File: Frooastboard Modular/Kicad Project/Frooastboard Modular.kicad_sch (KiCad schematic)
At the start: 41 parts, among them J1 Conn_01x08, J2 Conn_01x06, J3 Conn_01x06, J4 Conn_01x10, J5 Conn_01x12, J6 SW Interface, J7 Conn_01x04, J8 Conn_01x08, U1 IS31FL3733-QF, U2 RP2040, U3 W25Q32JVZP, U4 LM317L_SOT-89, Y1 12MHz

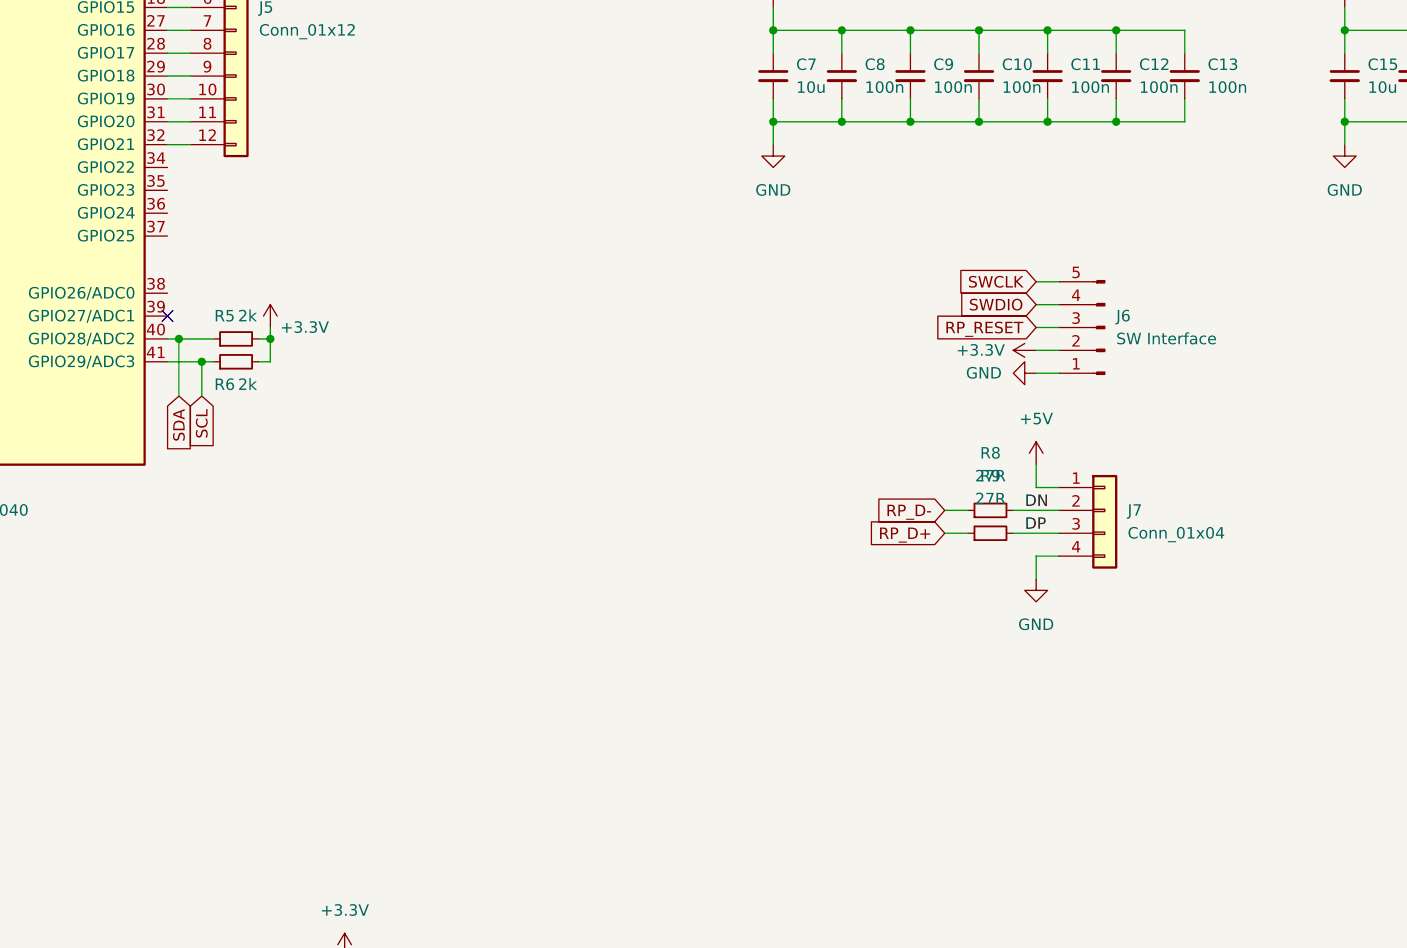
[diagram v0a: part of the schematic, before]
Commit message: before moving stuff
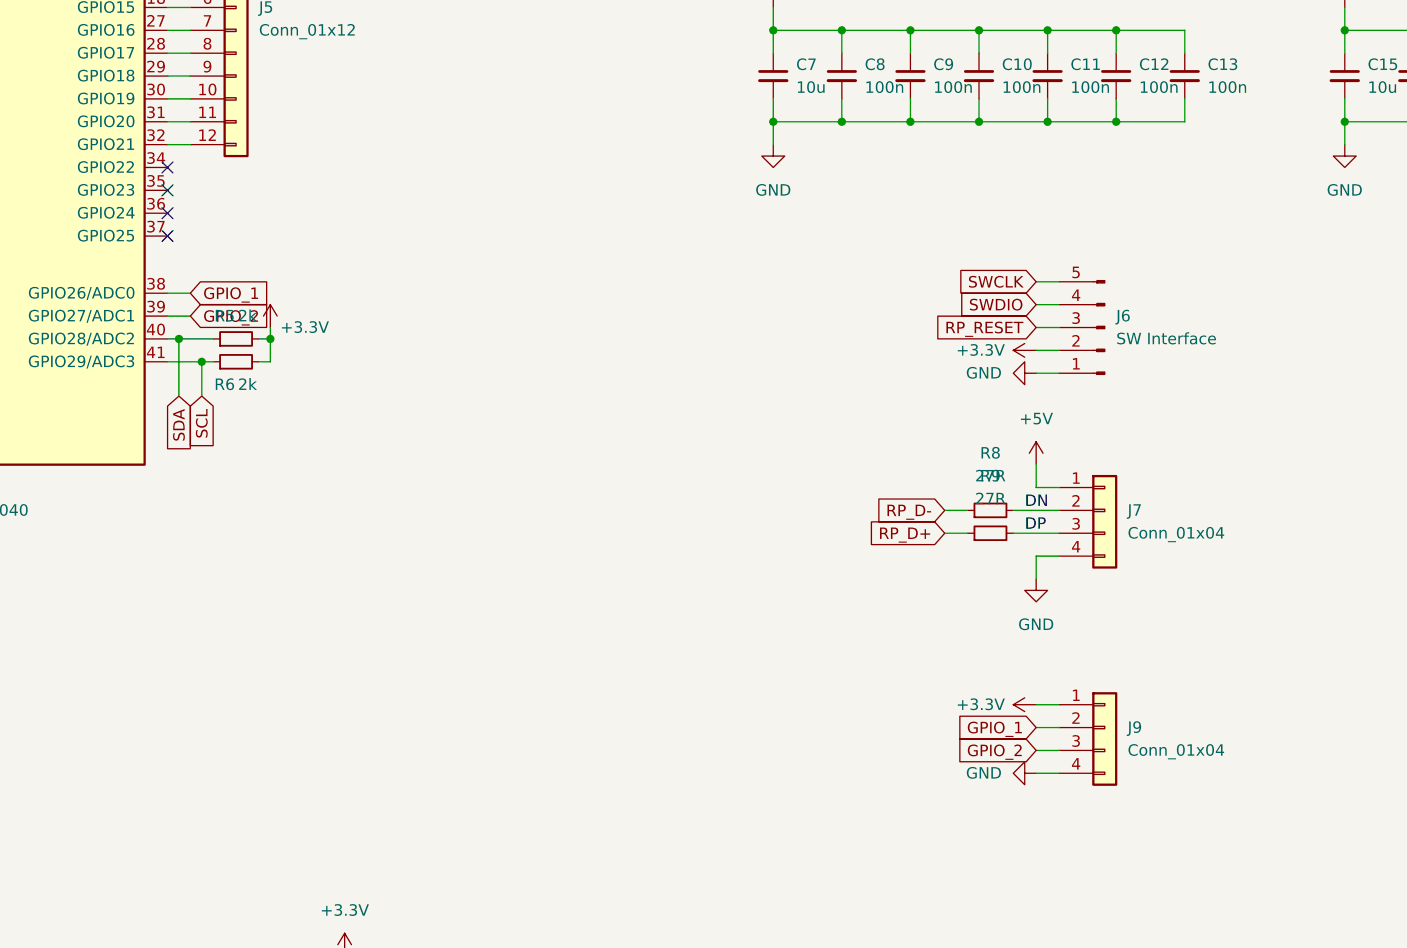
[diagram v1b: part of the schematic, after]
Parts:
- added J9: Conn_01x04, Frooastboard Footprints:PinHeader_1x04_P1.27mm_Vertical, symbol Connector_Generic:Conn_01x04
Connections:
- net +3V3: now also J9.1 (Pin_1)
- net GND: now also J9.4 (Pin_4)
- net GPIO_1: now reaches U2.38 (GPIO26/ADC0)
- net GPIO_1: now also J9.2 (Pin_2)
- net GPIO_2: now reaches U2.39 (GPIO27/ADC1)
- net GPIO_2: now also J9.3 (Pin_3)
- no-connect marks 3 -> 6
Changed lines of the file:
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@@
   (junction (at 203.2 29.21) (diameter 0) (color 0 0 0 0)
   )
+  (no_connect (at 90.17 95.25))
   (no_connect (at 48.26 199.39))
-  (no_connect (at 90.17 109.22))
+  (no_connect (at 90.17 97.79))
+  (no_connect (at 90.17 100.33))
+  (no_connect (at 90.17 92.71))
   (no_connect (at 48.26 209.55))
   (wire (pts (xy 138.43 40.64) (xy 135.89 40.64))
@@
     (stroke (width 0) (type default))
   )
+  (wire (pts (xy 90.17 106.68) (xy 92.71 106.68))
+    (stroke (width 0) (type default))
+  )
   (wire (pts (xy 66.04 128.27) (xy 66.04 130.81))
     (stroke (width 0) (type default))
@@
     (stroke (width 0) (type default))
   )
+  (wire (pts (xy 90.17 109.22) (xy 92.71 109.22))
+    (stroke (width 0) (type default))
+  )
   (wire (pts (xy 261.62 36.83) (xy 261.62 39.37))
     (stroke (width 0) (type default))
@@
     (stroke (width 0) (type default))
   )
+  (wire (pts (xy 186.69 157.48) (xy 189.23 157.48))
+    (stroke (width 0) (type default))
+  )
   (wire (pts (xy 66.04 267.97) (xy 66.04 265.43))
     (stroke (width 0) (type default))
@@
     (stroke (width 0) (type default))
   )
+  (wire (pts (xy 186.69 160.02) (xy 189.23 160.02))
+    (stroke (width 0) (type default))
+  )
   (wire (pts (xy 123.825 193.04) (xy 133.985 193.04))
     (stroke (width 0) (type default))
@@
     (stroke (width 0) (type default))
   )
+  (wire (pts (xy 186.69 154.94) (xy 189.23 154.94))
+    (stroke (width 0) (type default))
+  )
   (wire (pts (xy 135.89 40.64) (xy 135.89 43.18))
     (stroke (width 0) (type default))
@@
     (stroke (width 0) (type default))
   )
+  (wire (pts (xy 186.69 152.4) (xy 189.23 152.4))
+    (stroke (width 0) (type default))
+  )
   (wire (pts (xy 261.62 39.37) (xy 264.16 39.37))
     (stroke (width 0) (type default))
@@
     )
   )
+  (global_label "GPIO_1" (shape input) (at 186.69 154.94 180) (fields_autoplaced)
+    (effects (font (size 1.27 1.27)) (justify right))
+    (property "Intersheetrefs" "${INTERSHEET_REFS}" (at 177.1318 154.94 0)
+      (effects (font (size 1.27 1.27)) (justify right) hide)
+    )
+  )
   (global_label "QSPI_SD0" (shape input) (at 46.99 104.14 180) (fields_autoplaced)
     (effects (font (size 1.27 1.27)) (justify right))
@@
     )
   )
+  (global_label "GPIO_1" (shape input) (at 92.71 106.68 0) (fields_autoplaced)
+    (effects (font (size 1.27 1.27)) (justify left))
+    (property "Intersheetrefs" "${INTERSHEET_REFS}" (at 102.2682 106.68 0)
+      (effects (font (size 1.27 1.27)) (justify left) hide)
+    )
+  )
   (global_label "SWDIO" (shape input) (at 46.99 93.98 180) (fields_autoplaced)
     (effects (font (size 1.27 1.27)) (justify right))
@@
     )
   )
+  (global_label "GPIO_2" (shape input) (at 92.71 109.22 0) (fields_autoplaced)
+    (effects (font (size 1.27 1.27)) (justify left))
+    (property "Intersheetrefs" "${INTERSHEET_REFS}" (at 102.2682 109.22 0)
+      (effects (font (size 1.27 1.27)) (justify left) hide)
+    )
+  )
   (global_label "QSPI_SD3" (shape input) (at 46.99 111.76 180) (fields_autoplaced)
     (effects (font (size 1.27 1.27)) (justify right))
@@
     )
   )
+  (global_label "GPIO_2" (shape input) (at 186.69 157.48 180) (fields_autoplaced)
+    (effects (font (size 1.27 1.27)) (justify right))
+    (property "Intersheetrefs" "${INTERSHEET_REFS}" (at 177.1318 157.48 0)
+      (effects (font (size 1.27 1.27)) (justify right) hide)
+    )
+  )
   (global_label "SDA" (shape input) (at 45.72 194.31 180) (fields_autoplaced)
     (effects (font (size 1.27 1.27)) (justify right))
@@
     )
   )
+  (symbol (lib_id "power:GND") (at 186.69 160.02 270) (unit 1)
+    (in_bom yes) (on_board yes) (dnp no) (fields_autoplaced)
+    (property "Reference" "#PWR032" (at 180.34 160.02 0)
+      (effects (font (size 1.27 1.27)) hide)
+    )
+    (property "Value" "GND" (at 182.88 160.0199 90)
+      (effects (font (size 1.27 1.27)) (justify right))
+    )
+    (property "Footprint" "" (at 186.69 160.02 0)
+      (effects (font (size 1.27 1.27)) hide)
+    )
+    (property "Datasheet" "" (at 186.69 160.02 0)
+      (effects (font (size 1.27 1.27)) hide)
+    )
+    (pin "1")
+    (instances
+      (project "Frooastboard Modular"
+        (path "/9ee55997-d93e-462c-b474-dae14d38ea26"
+          (reference "#PWR032") (unit 1)
+        )
+      )
+      (project "Frooastboard Walnut Modular"
+        (path "/e63e39d7-6ac0-4ffd-8aa3-1841a4541b55"
+          (reference "#PWR0120") (unit 1)
+        )
+        (path "/e63e39d7-6ac0-4ffd-8aa3-1841a4541b55/eba7bed6-3b4a-4b7a-b4a2-784017f24fe8"
+          (reference "#PWR020") (unit 1)
+        )
+      )
+    )
+  )
   (symbol (lib_id "Device:R_Small") (at 97.79 111.76 90) (unit 1)
     (in_bom yes) (on_board yes) (dnp no)
@@
     )
   )
+  (symbol (lib_id "Connector_Generic:Conn_01x04") (at 194.31 154.94 0) (unit 1)
+    (in_bom yes) (on_board yes) (dnp no) (fields_autoplaced)
+    (property "Reference" "J9" (at 196.85 154.94 0)
+      (effects (font (size 1.27 1.27)) (justify left))
+    )
+    (property "Value" "Conn_01x04" (at 196.85 157.48 0)
+      (effects (font (size 1.27 1.27)) (justify left))
+    )
+    (property "Footprint" "Frooastboard Footprints:PinHeader_1x04_P1.27mm_Vertical" (at 194.31 154.94 0)
+      (effects (font (size 1.27 1.27)) hide)
+    )
+    (property "Datasheet" "~" (at 194.31 154.94 0)
+      (effects (font (size 1.27 1.27)) hide)
+    )
+    (pin "1")
+    (pin "2")
+    (pin "3")
+    (pin "4")
+    (instances
+      (project "Frooastboard Modular"
+        (path "/9ee55997-d93e-462c-b474-dae14d38ea26"
+          (reference "J9") (unit 1)
+        )
+      )
+    )
+  )
   (symbol (lib_id "power:+3.3V") (at 109.855 180.34 0) (unit 1)
     (in_bom yes) (on_board yes) (dnp no) (fields_autoplaced)
@@
         )
       )
+    )
+  )
+  (symbol (lib_id "power:+3.3V") (at 186.69 152.4 90) (unit 1)
+    (in_bom yes) (on_board yes) (dnp no)
+    (property "Reference" "#PWR031" (at 190.5 152.4 0)
+      (effects (font (size 1.27 1.27)) hide)
+    )
+    (property "Value" "+3.3V" (at 177.8 152.4 90)
+      (effects (font (size 1.27 1.27)) (justify right))
+    )
+    (property "Footprint" "" (at 186.69 152.4 0)
+      (effects (font (size 1.27 1.27)) hide)
+    )
+    (property "Datasheet" "" (at 186.69 152.4 0)
+      (effects (font (size 1.27 1.27)) hide)
+    )
+    (pin "1")
+    (instances
+      (project "Frooastboard Modular"
+        (path "/9ee55997-d93e-462c-b474-dae14d38ea26"
+          (reference "#PWR031") (unit 1)
+        )
+      )
+      (project "Frooastboard Walnut Modular"
+        (path "/e63e39d7-6ac0-4ffd-8aa3-1841a4541b55"
+          (reference "#PWR0119") (unit 1)
+        )
+        (path "/e63e39d7-6ac0-4ffd-8aa3-1841a4541b55/eba7bed6-3b4a-4b7a-b4a2-784017f24fe8"
+          (reference "#PWR019") (unit 1)
+        )
+      )

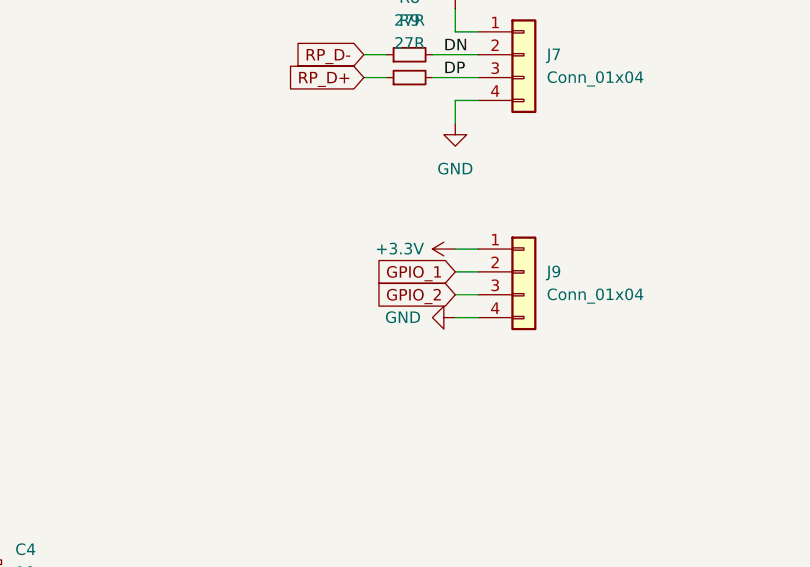
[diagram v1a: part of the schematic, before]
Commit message: somewhat good
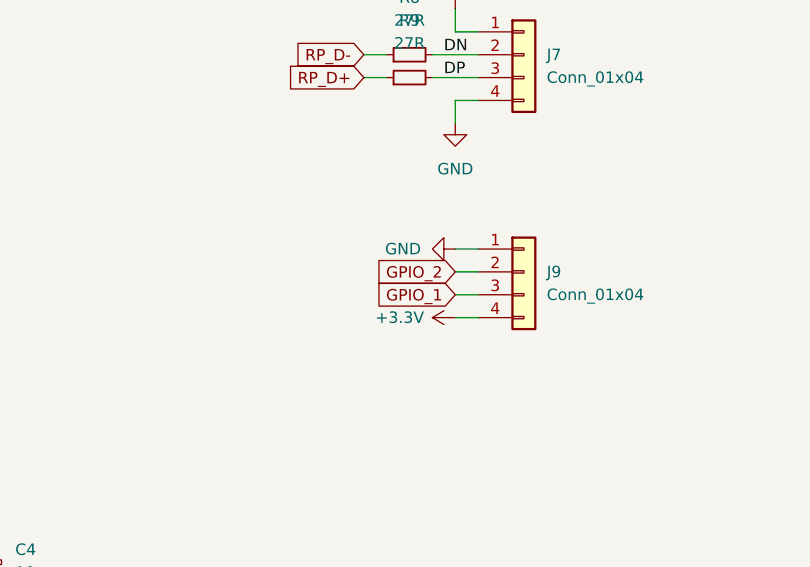
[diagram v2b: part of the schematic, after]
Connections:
- net +3V3: now also J9.4 (Pin_4); no longer J9.1 (Pin_1)
- net GND: now also J9.1 (Pin_1); no longer J9.4 (Pin_4)
- net GPIO_1: now also J9.3 (Pin_3); no longer J9.2 (Pin_2)
- net GPIO_2: now also J9.2 (Pin_2); no longer J9.3 (Pin_3)
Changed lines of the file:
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@@
     )
   )
-  (global_label "GPIO_1" (shape input) (at 186.69 154.94 180) (fields_autoplaced)
+  (global_label "GPIO_1" (shape input) (at 186.69 157.48 180) (fields_autoplaced)
     (effects (font (size 1.27 1.27)) (justify right))
-    (property "Intersheetrefs" "${INTERSHEET_REFS}" (at 177.1318 154.94 0)
+    (property "Intersheetrefs" "${INTERSHEET_REFS}" (at 177.1318 157.48 0)
       (effects (font (size 1.27 1.27)) (justify right) hide)
     )
@@
     )
   )
-  (global_label "GPIO_2" (shape input) (at 186.69 157.48 180) (fields_autoplaced)
+  (global_label "GPIO_2" (shape input) (at 186.69 154.94 180) (fields_autoplaced)
     (effects (font (size 1.27 1.27)) (justify right))
-    (property "Intersheetrefs" "${INTERSHEET_REFS}" (at 177.1318 157.48 0)
+    (property "Intersheetrefs" "${INTERSHEET_REFS}" (at 177.1318 154.94 0)
       (effects (font (size 1.27 1.27)) (justify right) hide)
     )
@@
     )
   )
-  (symbol (lib_id "power:GND") (at 186.69 160.02 270) (unit 1)
-    (in_bom yes) (on_board yes) (dnp no) (fields_autoplaced)
-    (property "Reference" "#PWR032" (at 180.34 160.02 0)
-      (effects (font (size 1.27 1.27)) hide)
-    )
-    (property "Value" "GND" (at 182.88 160.0199 90)
+  (symbol (lib_id "power:GND") (at 186.69 152.4 270) (unit 1)
+    (in_bom yes) (on_board yes) (dnp no) (fields_autoplaced)
+    (property "Reference" "#PWR032" (at 180.34 152.4 0)
+      (effects (font (size 1.27 1.27)) hide)
+    )
+    (property "Value" "GND" (at 182.88 152.3999 90)
       (effects (font (size 1.27 1.27)) (justify right))
     )
-    (property "Footprint" "" (at 186.69 160.02 0)
-      (effects (font (size 1.27 1.27)) hide)
-    )
-    (property "Datasheet" "" (at 186.69 160.02 0)
+    (property "Footprint" "" (at 186.69 152.4 0)
+      (effects (font (size 1.27 1.27)) hide)
+    )
+    (property "Datasheet" "" (at 186.69 152.4 0)
       (effects (font (size 1.27 1.27)) hide)
     )
@@
     )
   )
-  (symbol (lib_id "power:+3.3V") (at 186.69 152.4 90) (unit 1)
+  (symbol (lib_id "power:+3.3V") (at 186.69 160.02 90) (unit 1)
     (in_bom yes) (on_board yes) (dnp no)
-    (property "Reference" "#PWR031" (at 190.5 152.4 0)
-      (effects (font (size 1.27 1.27)) hide)
-    )
-    (property "Value" "+3.3V" (at 177.8 152.4 90)
+    (property "Reference" "#PWR031" (at 190.5 160.02 0)
+      (effects (font (size 1.27 1.27)) hide)
+    )
+    (property "Value" "+3.3V" (at 177.8 160.02 90)
       (effects (font (size 1.27 1.27)) (justify right))
     )
-    (property "Footprint" "" (at 186.69 152.4 0)
-      (effects (font (size 1.27 1.27)) hide)
-    )
-    (property "Datasheet" "" (at 186.69 152.4 0)
-      (effects (font (size 1.27 1.27)) hide)
-    )
+    (property "Footprint" "" (at 186.69 160.02 0)
+      (effects (font (size 1.27 1.27)) hide)
+    )
+    (property "Datasheet" "" (at 186.69 160.02 0)
+      (effects (font (size 1.27 1.27)) hide)
+    )
